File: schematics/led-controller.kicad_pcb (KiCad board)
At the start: 2 copper layers, 58 parts, among them IC1 ATMEGA168A-P, P1 CONN_01X03, P2 CONN_01X03, P3 CONN_01X02, P4 CONN_01X02, P5 CONN_01X02, P6 CONN_01X02, P7 ISP, P8 COM, Q1 IRLU 120N, Q2 IRLU 120N, Q3 IRLU 120N, Q4 IRLU 120N, U1 LM339, U2 74HCT04_3V3, U3 LF33CV, U4 74HC08_3V3

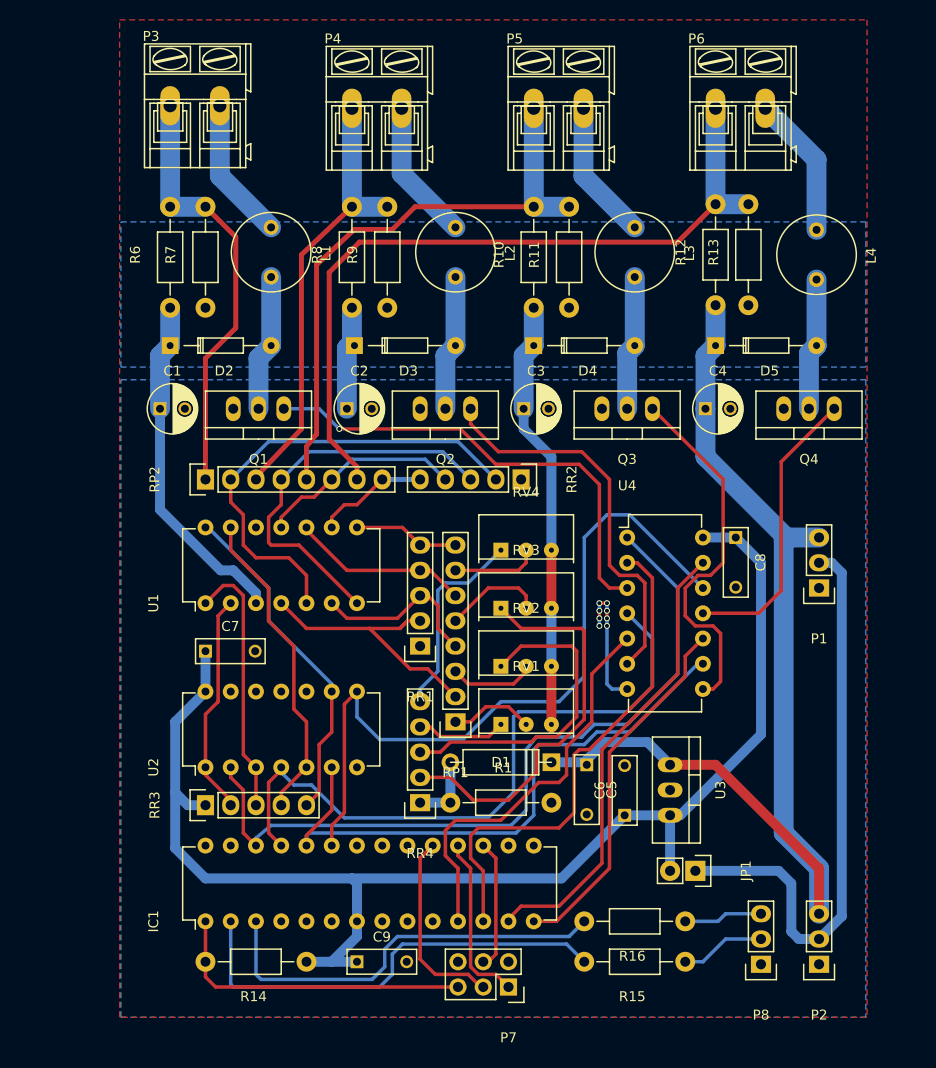
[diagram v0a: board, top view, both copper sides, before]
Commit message: first checked version
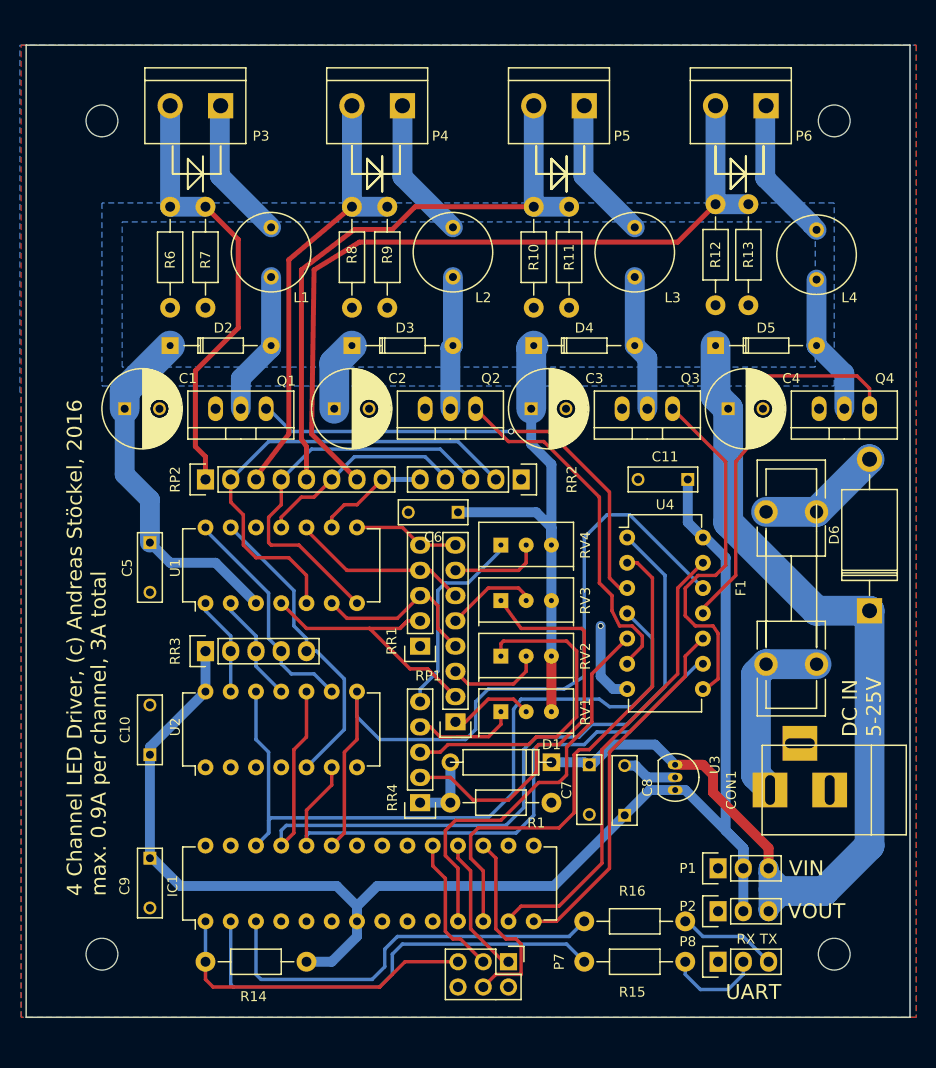
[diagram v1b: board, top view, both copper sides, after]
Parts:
- removed JP1: Jumper_NO_Small, Pin_Headers:Pin_Header_Straight_1x02
- added C10: 100n, Capacitors_ThroughHole:C_Rect_L7_W2.5_P5, F.Cu at (103.9, 101.9)
- added C11: 100n, Capacitors_ThroughHole:C_Rect_L7_W2.5_P5, F.Cu at (158.0, 74.2)
- added CON1: BARREL_JACK, Connect:BARREL_JACK, F.Cu at (172.5, 105.4)
- added D6: 1N5408, Diodes_ThroughHole:Diode_DO-201AD_Horizontal_RM15, F.Cu at (176.3, 87.4)
- added F1: 3A, Fuse_Holders_and_Fuses:Fuseholder5x20_horiz_open_lateral_Type-II, F.Cu at (168.4, 85.1)
- added REF**: MountingHole_3.2mm_M3, Mounting_Holes:MountingHole_3.2mm_M3, F.Cu at (99.1, 121.9)
- added REF**: MountingHole_3.2mm_M3, Mounting_Holes:MountingHole_3.2mm_M3, F.Cu at (99.1, 38.1)
- added REF**: MountingHole_3.2mm_M3, Mounting_Holes:MountingHole_3.2mm_M3, F.Cu at (172.7, 38.1)
- added REF**: MountingHole_3.2mm_M3, Mounting_Holes:MountingHole_3.2mm_M3, F.Cu at (172.7, 121.9)
- C1, C2, C3, C4: footprint Capacitors_ThroughHole:C_Radial_D5_L11_P2.5 -> Capacitors_ThroughHole:C_Radial_D8_L11.5_P3.5
- P1: value CONN_01X03 -> VIN
- P2: value CONN_01X03 -> VOUT
- P3: value CONN_01X02 -> LED1; footprint Connect:AK300-2 -> Connect:bornier2
- P4, P5, P6: footprint Connect:AK300-2 -> Connect:bornier2
- P7: footprint Socket_Strips:Socket_Strip_Straight_2x03 -> Pin_Headers:Pin_Header_Straight_2x03
- RR4: value 20k -> 27k
- RV1, RV2, RV3, RV4: footprint Potentiometers:Potentiometer_Trimmer-Suntan-TSR-3386C -> Trimmers:Potentiometer_Trimmer-Suntan-TSR-3296
- U3: value LF33CV -> LP 2950 ACZ3,3; footprint TO_SOT_Packages_THT:TO-220_Neutral123_Vertical -> TO_SOT_Packages_THT:TO-92_Inline_Narrow_Oval
- moved C5 49.3 mm to (103.9, 80.5)
- moved C7 40.3 mm to (148.1, 102.9), turned to 270 degrees
- moved C6 34.8 mm to (134.9, 77.5), turned to 180 degrees
- moved P1 34.1 mm to (161.0, 117.6), turned to 90 degrees
- moved C8 30.1 mm to (151.6, 108.0), turned to 90 degrees
- moved C9 23.3 mm to (103.9, 112.3), turned to 270 degrees
- moved RR3 15.5 mm to (109.5, 91.4)
- moved P2 14.0 mm to (161.0, 113.3), turned to 90 degrees
- moved P8 4.33 mm to (161.0, 122.7), turned to 90 degrees
- moved C1 3.56 mm to (101.3, 67.1)
- moved Q4 3.56 mm to (173.7, 67.1)
- moved U3 2.59 mm to (156.7, 102.9)
- moved P4 2.55 mm to (126.7, 36.6), turned to 180 degrees
- moved P5 2.55 mm to (145.0, 36.6), turned to 180 degrees
- moved P6 2.55 mm to (163.3, 36.6), turned to 180 degrees
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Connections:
- C6 pad 1: +3V3 -> VCC
- C7 pad 1: +3V3 -> VCC
- IC1 pad 25: SENSE2 -> SENSE1
- IC1 pad 26: SENSE1 -> SENSE2
- P1 pad 2: Net-(JP1-Pad1) -> +3V3
- P2 pad 2: Net-(JP1-Pad1) -> +3V3
- P3 pad 1: /IRAW1 -> Net-(L1-Pad1)
- P3 pad 2: Net-(L1-Pad1) -> /IRAW1
- P4 pad 1: /IRAW2 -> Net-(L2-Pad1)
- P4 pad 2: Net-(L2-Pad1) -> /IRAW2
- P5 pad 1: /IRAW3 -> Net-(L3-Pad1)
- P5 pad 2: Net-(L3-Pad1) -> /IRAW3
- P6 pad 1: /IRAW4 -> Net-(L4-Pad1)
- P6 pad 2: Net-(L4-Pad1) -> /IRAW4
- RR3 pad 2: /PULLUP1 -> /PULLUP2
- RR3 pad 3: /PULLUP2 -> /PULLUP1
- RR3 pad 4: /PULLUP3 -> /PULLUP4
- RR3 pad 5: /PULLUP4 -> /PULLUP3
- U2 pad 1: /PULLUP1 -> (no net)
- U2 pad 10: (no net) -> SENSE1
- U2 pad 11: (no net) -> /PULLUP1
- U2 pad 12: (no net) -> SENSE2
- U2 pad 13: (no net) -> /PULLUP2
- U2 pad 2: SENSE1 -> (no net)
- U2 pad 3: /PULLUP2 -> (no net)
- U2 pad 4: SENSE2 -> (no net)
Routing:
- net Net-(JP1-Pad1): track 58.6 -> 0.00 mm
- net Net-(CON1-Pad1): track 0.00 -> 18.7 mm
- net +3V3: track 135.3 -> 152.8 mm
- net /PULLUP2: track 26.6 -> 9.94 mm
- net Net-(D6-Pad2): track 0.00 -> 12.6 mm
- net /PULLUP1: track 22.4 -> 11.0 mm
- net /PULLUP4: track 34.4 -> 23.1 mm
- net SWITCH4: track 29.3 -> 39.5 mm
- net SENSE2: track 67.3 -> 76.0 mm
- net MOSI: track 12.8 -> 19.5 mm
- net VCC: track 197.5 -> 203.0 mm
- net SCK: track 19.5 -> 14.2 mm
- net SENSE1: track 78.4 -> 82.9 mm
- net SWITCH2: track 39.6 -> 35.9 mm
- net MISO: track 17.6 -> 14.1 mm
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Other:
- board outline added: 88.9 x 97.8 mm
- board text added: "4 Channel LED Driver, (c) Andreas Stöckel, 2016 max. 0.9A per channel, 3A total"
- board text added: "DC IN 5-25V"
- board text added: "RX"
- board text added: "TX"
- board text added: "UART"
- board text added: "VIN"
- board text added: "VOUT"
